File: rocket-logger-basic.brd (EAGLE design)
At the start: 58.5 x 62 mm, 61 parts, among them IC1 CC430F513X, Q2 MOSFET-PCHANNEL, U2 MAX1555, U3 MCP73831, X1 0896BM15A0001, X2 USB-MICROB, X3 SMA-142-0701-801/806

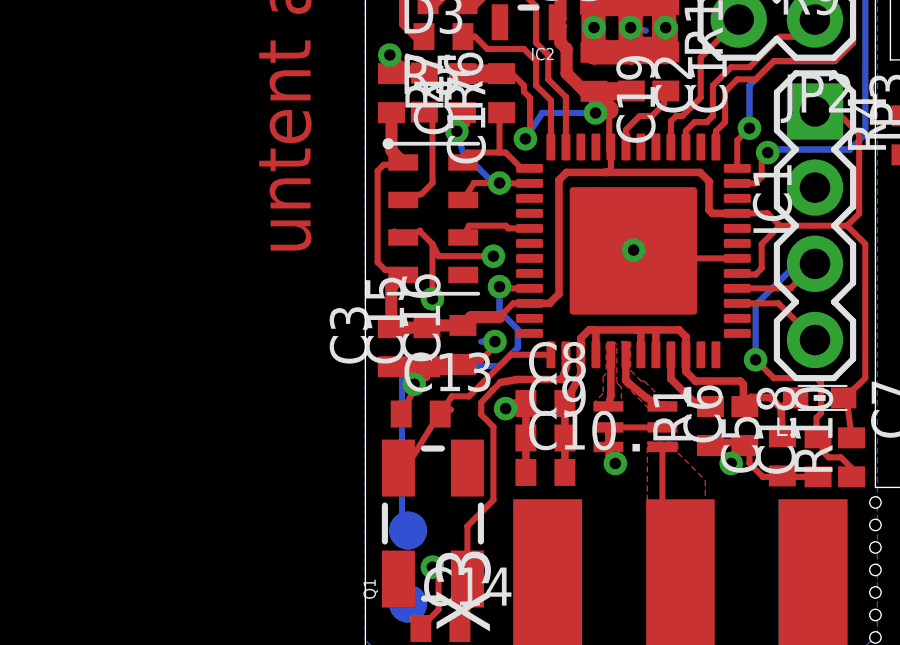
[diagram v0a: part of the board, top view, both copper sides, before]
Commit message: fixing some drc
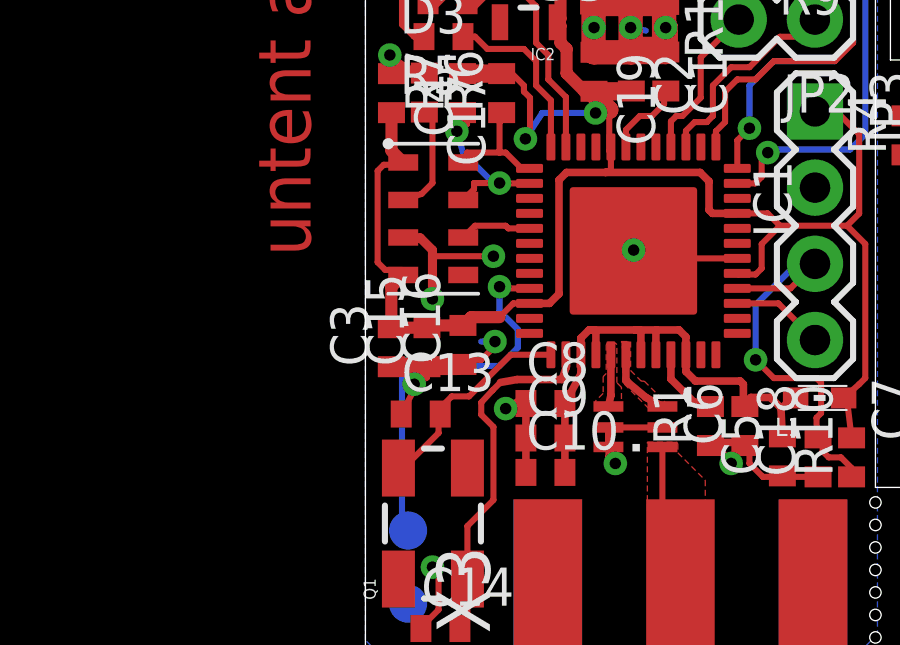
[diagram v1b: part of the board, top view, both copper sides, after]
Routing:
- net GND: track 72.8 -> 71.9 mm
- net N$6: track 7.68 -> 7.07 mm
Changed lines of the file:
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@@
 <setting verticaltext="up"/>
 </settings>
-<grid distance="8" unitdist="mil" unit="mil" style="dots" multiple="1" display="no" altdistance="2" altunitdist="mil" altunit="mm"/>
+<grid distance="8" unitdist="mil" unit="mil" style="dots" multiple="1" display="yes" altdistance="2" altunitdist="mil" altunit="mm"/>
 <layers>
 <layer number="1" name="Top" color="4" fill="1" visible="yes" active="yes"/>
@@
 <layer number="49" name="Reference" color="7" fill="1" visible="no" active="yes"/>
 <layer number="50" name="dxf" color="7" fill="1" visible="no" active="no"/>
-<layer number="51" name="tDocu" color="6" fill="1" visible="no" active="yes"/>
+<layer number="51" name="tDocu" color="6" fill="1" visible="yes" active="yes"/>
 <layer number="52" name="bDocu" color="3" fill="1" visible="no" active="yes"/>
 <layer number="53" name="tPadExt" color="7" fill="1" visible="no" active="no"/>
@@
 <layer number="109" name="ref-old" color="11" fill="1" visible="no" active="yes"/>
 <layer number="116" name="Patch_BOT" color="9" fill="4" visible="no" active="yes"/>
-<layer number="121" name="_tsilk" color="7" fill="1" visible="yes" active="yes"/>
-<layer number="122" name="_bsilk" color="7" fill="1" visible="yes" active="yes"/>
+<layer number="121" name="_tsilk" color="7" fill="1" visible="no" active="yes"/>
+<layer number="122" name="_bsilk" color="7" fill="1" visible="no" active="yes"/>
 <layer number="125" name="_tNames" color="7" fill="1" visible="no" active="yes"/>
 <layer number="144" name="Drill_legend" color="7" fill="1" visible="no" active="yes"/>
@@
 <wire x1="11.5" y1="7" x2="12.65" y2="7" width="0.254" layer="1"/>
 <wire x1="12.65" y1="7" x2="12.6484" y2="6.8968" width="0.254" layer="1"/>
-<wire x1="1.26" y1="13.8318" x2="0.965" y2="14.035" width="0.2032" layer="1"/>
 <contactref element="C26" pad="1"/>
 <contactref element="TP2" pad="TP"/>
@@
 <wire x1="4.318" y1="10.3632" x2="3.8608" y2="10.3632" width="0.2032" layer="16"/>
 <via x="2.2352" y="11.7856" extent="1-16" drill="0.381" shape="octagon"/>
-<wire x1="1.26" y1="13.8318" x2="1.8146" y2="14.035" width="0.2032" layer="1"/>
-<wire x1="1.8146" y1="14.035" x2="2.2352" y2="13.6144" width="0.2032" layer="1"/>
-<wire x1="2.2352" y1="13.6144" x2="2.2352" y2="11.7856" width="0.2032" layer="1"/>
-<wire x1="1.8146" y1="14.035" x2="1.8146" y2="14.0646" width="0.2032" layer="1"/>
 <wire x1="1.9644" y1="19.3124" x2="1.2552" y2="19.3124" width="0.2032" layer="1"/>
 <wire x1="1.2552" y1="19.3124" x2="0.8684" y2="19.2928" width="0.2032" layer="1"/>
 <wire x1="2.2352" y1="19.3972" x2="1.9644" y2="19.3124" width="0.2032" layer="1"/>
 <via x="4.2672" y="13.208" extent="1-16" drill="0.381" shape="octagon"/>
-<wire x1="4.2672" y1="13.208" x2="2.4384" y2="13.208" width="0.2032" layer="1"/>
-<wire x1="2.4384" y1="13.208" x2="2.2352" y2="13.6144" width="0.2032" layer="1"/>
+<wire x1="4.2672" y1="13.208" x2="2.2352" y2="13.208" width="0.2032" layer="1"/>
 <via x="8.9408" y="13.4112" extent="1-16" drill="0.381" shape="octagon"/>
 <wire x1="8.9408" y1="13.4112" x2="8.9408" y2="13.3926" width="0.2032" layer="1"/>
@@
 <wire x1="7.9248" y1="30.8864" x2="7.9248" y2="31.2656" width="0.2032" layer="1"/>
 <wire x1="7.9248" y1="31.2656" x2="7.974" y2="31.3148" width="0.2032" layer="1"/>
+<wire x1="2.2352" y1="11.7856" x2="2.2352" y2="13.208" width="0.3048" layer="1"/>
+<wire x1="2.2352" y1="13.208" x2="2.2352" y2="13.4112" width="0.3048" layer="1"/>
+<wire x1="2.2352" y1="13.4112" x2="1.8288" y2="13.8176" width="0.3048" layer="1"/>
+<wire x1="1.8288" y1="13.8176" x2="1.2742" y2="13.8176" width="0.3048" layer="1"/>
+<wire x1="1.2742" y1="13.8176" x2="1.26" y2="13.8318" width="0.3048" layer="1"/>
 <wire x1="11.3404" y1="28.448" x2="33.8372" y2="44.832" width="0" layer="19" extent="1-1"/>
 <wire x1="14.9196" y1="2.5654" x2="14.9196" y2="2.5654" width="0" layer="19" extent="1-16"/>
@@
 <contactref element="IC1" pad="25"/>
 <wire x1="1.1" y1="6.1468" x2="1.4732" y2="6.35" width="0.2032" layer="1"/>
-<wire x1="1.4732" y1="6.35" x2="2.4384" y2="7.9248" width="0.2032" layer="1"/>
-<wire x1="2.4384" y1="7.9248" x2="2.8448" y2="8.0948" width="0.2032" layer="1"/>
-<wire x1="2.8448" y1="8.0948" x2="2.4936" y2="7.9468" width="0.2032" layer="1"/>
 <wire x1="6.1832" y1="9.9225" x2="4.8425" y2="9.9225" width="0.2032" layer="1"/>
 <wire x1="4.8425" y1="9.9225" x2="3.4544" y2="8.5344" width="0.2032" layer="1"/>
 <wire x1="3.4544" y1="8.5344" x2="2.878" y2="8.5344" width="0.2032" layer="1"/>
-<wire x1="2.878" y1="8.5344" x2="2.4936" y2="7.9468" width="0.2032" layer="1"/>
+<wire x1="1.4732" y1="6.35" x2="2.4384" y2="7.3152" width="0.2032" layer="1"/>
+<wire x1="2.4384" y1="7.3152" x2="2.4384" y2="7.8916" width="0.2032" layer="1"/>
+<wire x1="2.4384" y1="7.8916" x2="2.4936" y2="7.9468" width="0.2032" layer="1"/>
+<wire x1="2.878" y1="8.5344" x2="2.4936" y2="8.15" width="0.2032" layer="1"/>
+<wire x1="2.4936" y1="8.15" x2="2.4936" y2="7.9468" width="0.2032" layer="1"/>
 </signal>
 <signal name="N$7">
@@
 <wire x1="3.048" y1="17.3736" x2="3.2512" y2="16.6624" width="0.2032" layer="16"/>
 <contactref element="IC1" pad="14"/>
-<wire x1="3.6214" y1="15.6464" x2="3.26" y2="15.0818" width="0.2032" layer="1"/>
 <wire x1="5.4707" y1="15.635" x2="4.4818" y2="15.635" width="0.2032" layer="1"/>
 <wire x1="4.4818" y1="15.635" x2="4.4704" y2="15.6464" width="0.2032" layer="1"/>
@@
 <wire x1="4.2672" y1="15.6464" x2="4.4704" y2="15.6464" width="0.2032" layer="16"/>
 <wire x1="3.6214" y1="15.6464" x2="4.4704" y2="15.6464" width="0.2032" layer="1"/>
+<wire x1="3.6214" y1="15.6464" x2="3.6214" y2="15.4432" width="0.2032" layer="1"/>
+<wire x1="3.6214" y1="15.4432" x2="3.26" y2="15.0818" width="0.2032" layer="1"/>
 </signal>
 <signal name="SCL">
@@
 <wire x1="5.4707" y1="14.135" x2="4.7626" y2="14.135" width="0.2032" layer="1"/>
 <wire x1="4.7626" y1="14.135" x2="4.6736" y2="14.224" width="0.2032" layer="1"/>
-<wire x1="4.6736" y1="14.224" x2="3.449" y2="14.224" width="0.2032" layer="1"/>
-<wire x1="3.449" y1="14.224" x2="3.26" y2="13.8318" width="0.2032" layer="1"/>
+<wire x1="4.6736" y1="14.224" x2="3.6522" y2="14.224" width="0.2032" layer="1"/>
+<wire x1="3.6522" y1="14.224" x2="3.26" y2="13.8318" width="0.2032" layer="1"/>
 </signal>
 <signal name="N$15">
